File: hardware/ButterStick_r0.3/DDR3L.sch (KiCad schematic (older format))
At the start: 2 parts, among them U4 MT41K64M16TW-107_J-TR

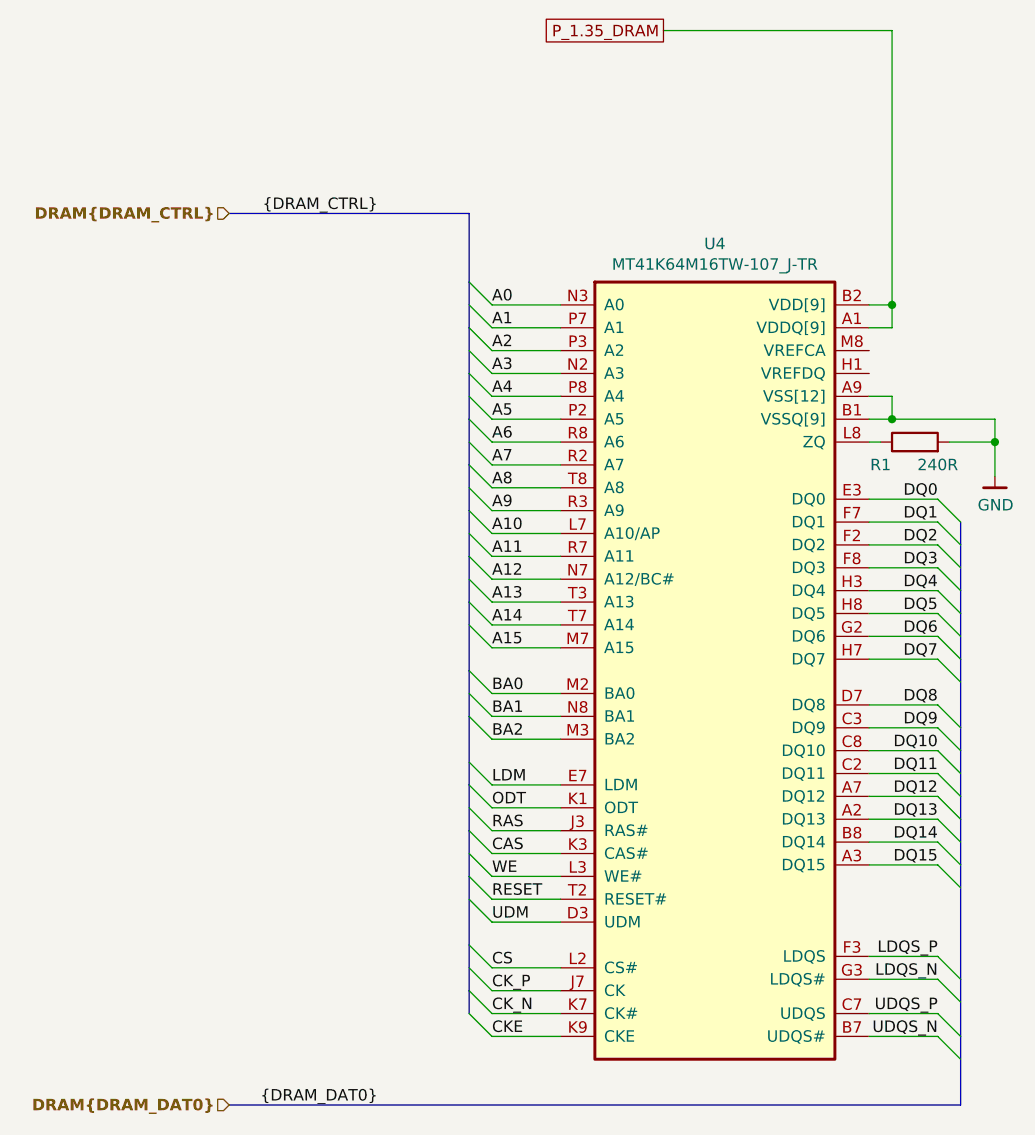
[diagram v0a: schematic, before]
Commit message: hw.r0_3: cleanup and additions
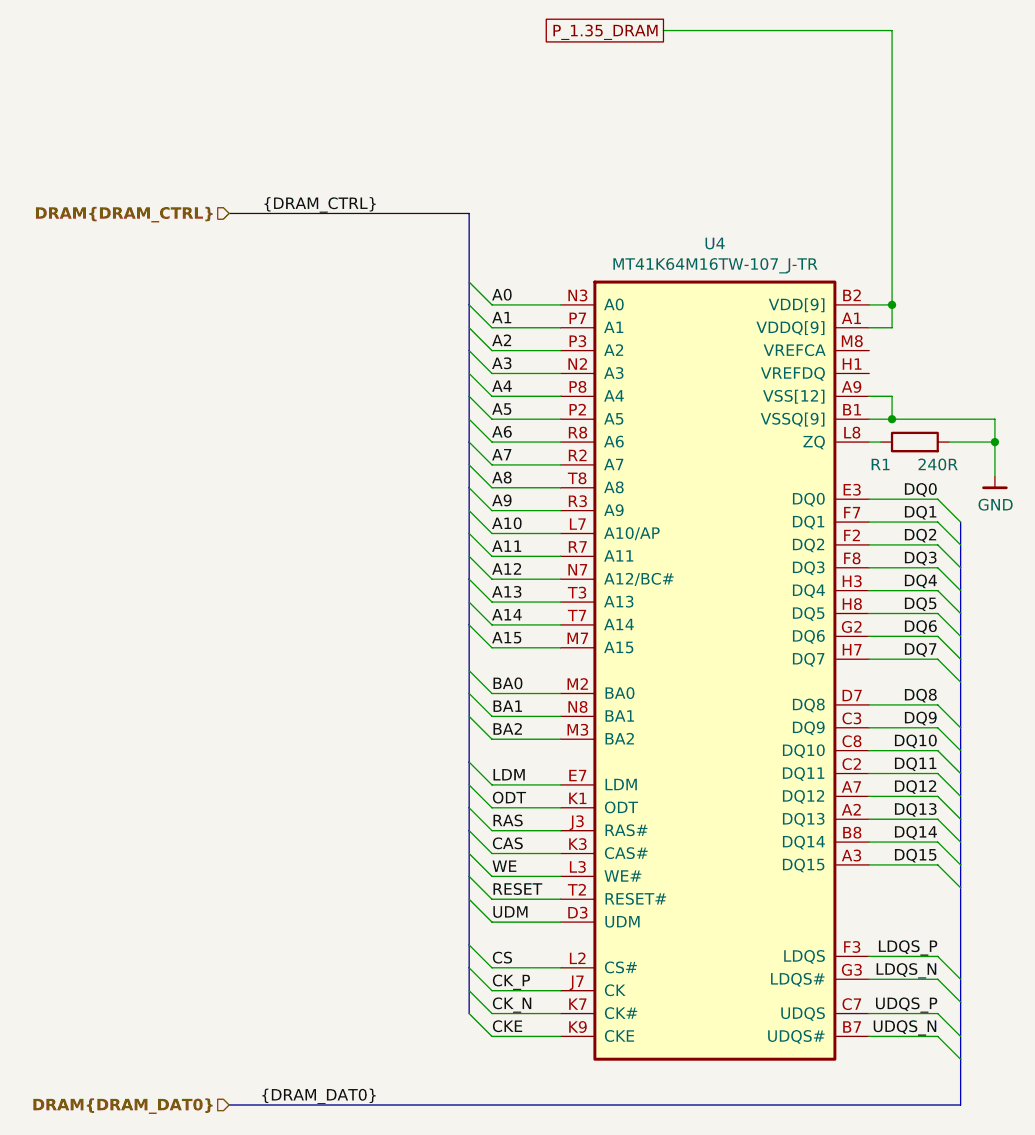
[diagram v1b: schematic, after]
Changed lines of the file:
@@
 $Descr A4 11693 8268
 encoding utf-8
-Sheet 6 16
+Sheet 14 20
 Title ""
 Date ""
@@
 	3300 6100 6500 6100
 Wire Bus Line
-	4350 2200 4350 2500
-Wire Bus Line
-	4350 2500 4350 2700
-Wire Bus Line
-	4350 2700 4350 2900
-Wire Bus Line
-	4350 2900 4350 3100
-Wire Bus Line
-	4350 3100 4350 3300
-Wire Bus Line
-	4350 3300 4350 3500
-Wire Bus Line
-	4350 3500 4350 3700
-Wire Bus Line
-	4350 3700 4350 3900
-Wire Bus Line
-	4350 3900 4350 4200
-Wire Bus Line
-	4350 4200 4350 4400
-Wire Bus Line
-	4350 4400 4350 4700
-Wire Bus Line
-	4350 4700 4350 4900
+	4350 2200 4350 2600
+Wire Bus Line
+	4350 2600 4350 2800
+Wire Bus Line
+	4350 2800 4350 3000
+Wire Bus Line
+	4350 3000 4350 3200
+Wire Bus Line
+	4350 3200 4350 3400
+Wire Bus Line
+	4350 3400 4350 3600
+Wire Bus Line
+	4350 3600 4350 3800
+Wire Bus Line
+	4350 3800 4350 4000
+Wire Bus Line
+	4350 4000 4350 4300
+Wire Bus Line
+	4350 4300 4350 4600
+Wire Bus Line
+	4350 4600 4350 4800
+Wire Bus Line
+	4350 4800 4350 4900
 Wire Bus Line
 	4350 4900 4350 5100
@@
 	4350 5100 4350 5400
 Wire Bus Line
-	4350 5400 4350 5600
-Wire Bus Line
-	4350 5600 4350 5700
-Wire Bus Line
-	6500 3550 6500 3650
-Wire Bus Line
-	6500 3650 6500 3850
-Wire Bus Line
-	6500 3850 6500 3950
+	4350 5400 4350 5500
+Wire Bus Line
+	4350 5500 4350 5700
+Wire Bus Line
+	6500 3550 6500 3750
+Wire Bus Line
+	6500 3750 6500 3950
 Wire Bus Line
 	6500 3950 6500 4150
@@
 	6500 4150 6500 4450
 Wire Bus Line
-	6500 4450 6500 4550
-Wire Bus Line
-	6500 4550 6500 4750
-Wire Bus Line
-	6500 4750 6500 4850
+	6500 4450 6500 4650
+Wire Bus Line
+	6500 4650 6500 4850
 Wire Bus Line
 	6500 4850 6500 5050
 Wire Bus Line
-	6500 5050 6500 5550
-Wire Bus Line
-	6500 5550 6500 5800
-Wire Bus Line
-	6500 5800 6500 6100
+	6500 5050 6500 5150
+Wire Bus Line
+	6500 5150 6500 5650
+Wire Bus Line
+	6500 5650 6500 5900
+Wire Bus Line
+	6500 5900 6500 6100
 Text Label 3950 2200 2    50   ~ 0
 {DRAM_CTRL}
